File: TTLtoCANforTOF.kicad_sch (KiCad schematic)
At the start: 47 parts, among them J2 CAN, J3 TOF, J4 XT30, J6 SWD, Q2 Si2309CDS-T1-GE3, U1 TPS54202DDC, U2 ME6211C33M5, U3 STM32G0B1CBTx, U6 TCAN3413DR, Y1 X32258MSB

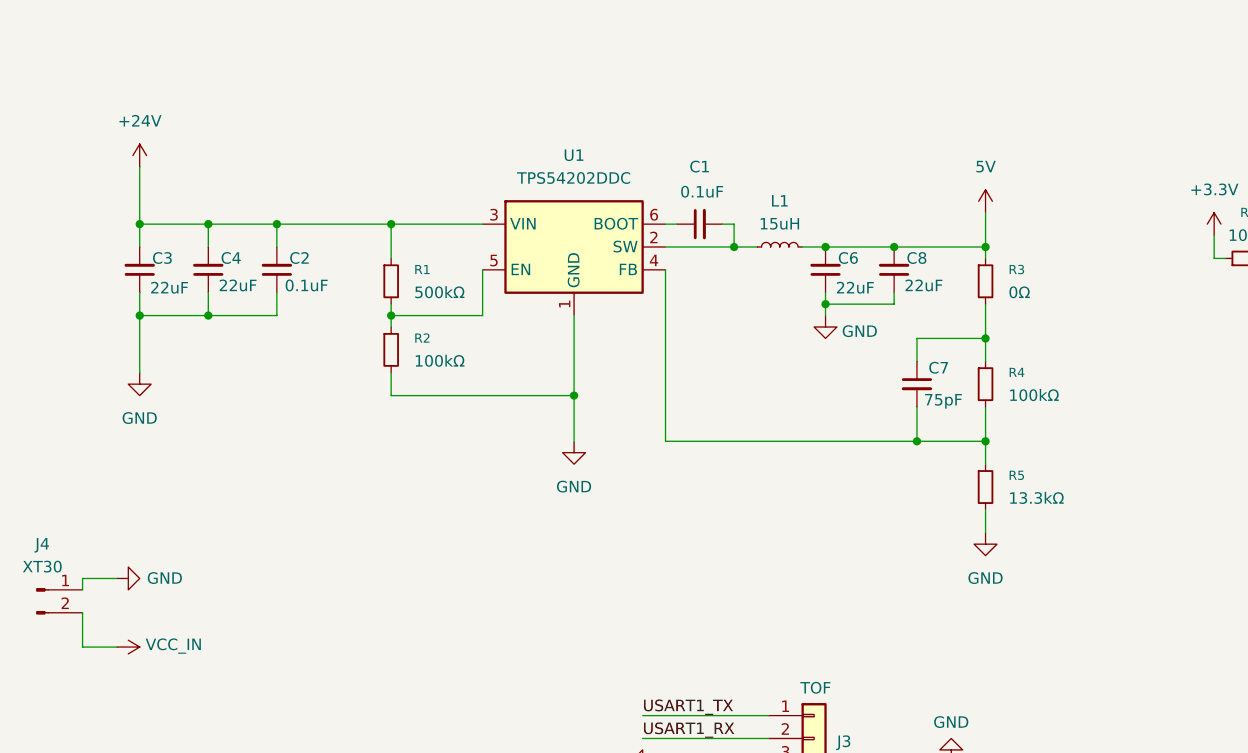
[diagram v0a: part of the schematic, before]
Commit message: fixbug
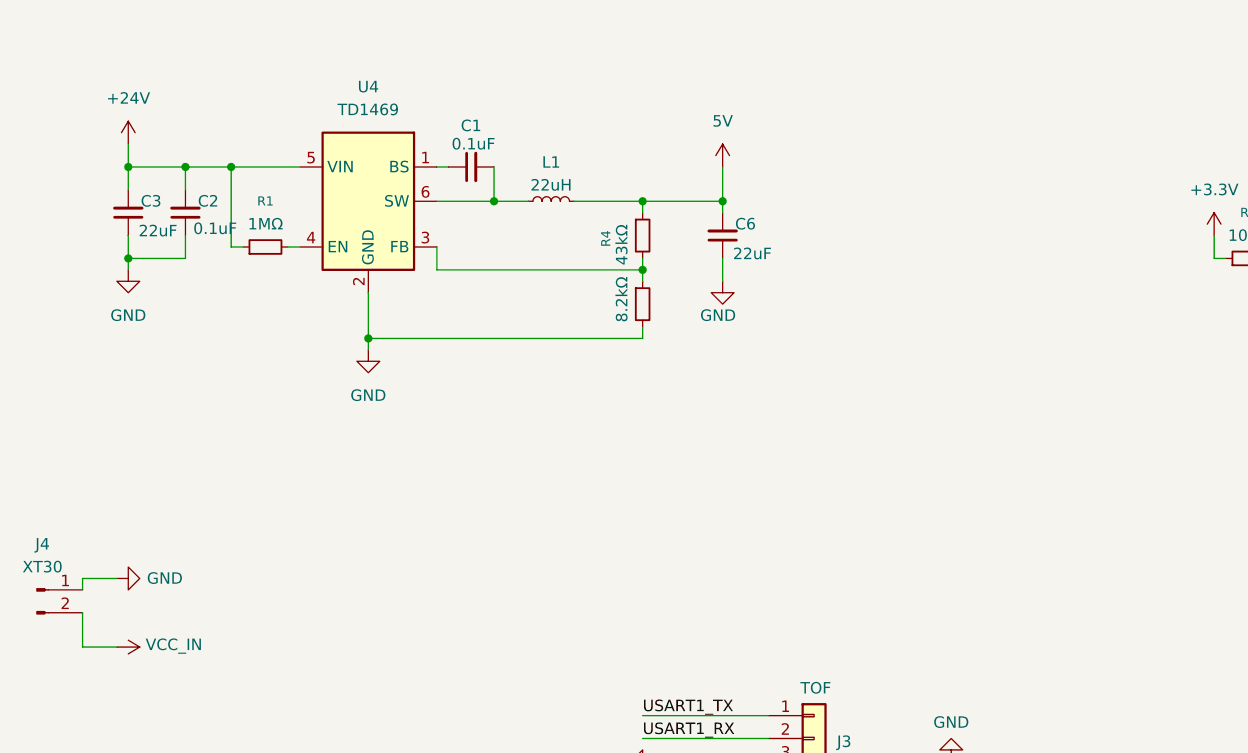
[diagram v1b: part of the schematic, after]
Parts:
- removed C4: 22uF, Capacitor_SMD:C_1210_3225Metric, symbol Device:C_Small
- removed C7: 75pF, Capacitor_SMD:C_0603_1608Metric, symbol Device:C_Small
- removed C8: 22uF, Capacitor_SMD:C_0805_2012Metric, symbol Device:C_Small
- removed R2: 100kΩ, Resistor_SMD:R_0603_1608Metric, symbol Device:R_Small
- removed R3: 0Ω, Resistor_SMD:R_0805_2012Metric, symbol Device:R_Small
- removed U1: TPS54202DDC, Package_TO_SOT_SMD:SOT-23-6, symbol Regulator_Switching:TPS54202DDC
- added U4: TD1469, Package_TO_SOT_SMD:SOT-23-6, symbol New_Library:TD1469
- L1: value 15uH -> 22uH
- R1: value 500kΩ -> 1MΩ
- R4: value 100kΩ -> 43kΩ
- R5: value 13.3kΩ -> 8.2kΩ
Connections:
- net +24V: now also U4.5 (VIN)
- net 5V: now also R4.1
- net GND: now also U4.2 (GND)
- net at R4.2, R5.1: now also U4.3 (FB)
- net at R1.2: now also U4.4 (EN)
- net at C1.1: now also U4.1 (BS)
- net at C1.2, L1.2: now also U4.6 (SW)
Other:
- moved on the sheet: C1, C3, C6, L1, R1, R4
